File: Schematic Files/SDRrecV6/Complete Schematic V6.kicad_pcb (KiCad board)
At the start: 2 copper layers, 99.6 x 99.7 mm, 74 parts, among them J1 Conn_Coaxial, J2 SJ1-3525N, U1 Si5351A-B-GT, U2 SN74CBT3253, U3 LT6231, U4 LM4562MA, Y1 Crystal_GND24_Small

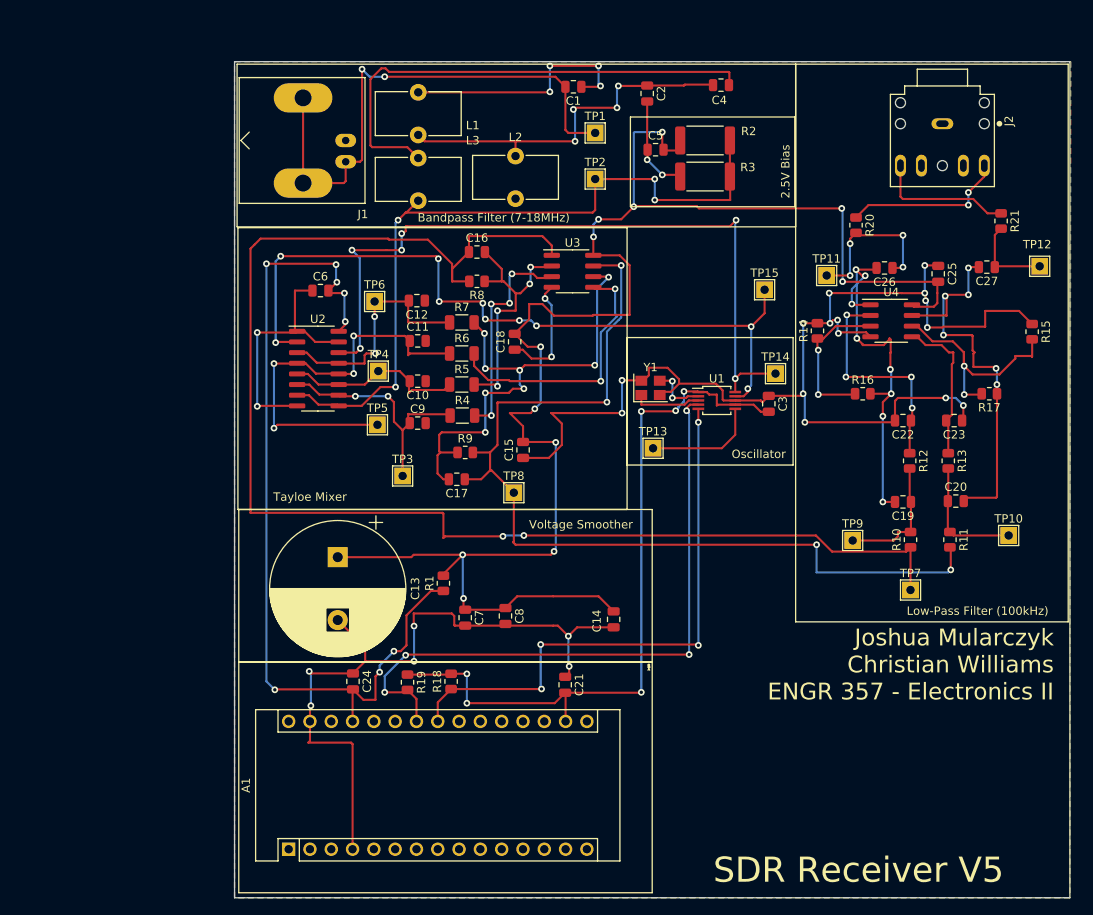
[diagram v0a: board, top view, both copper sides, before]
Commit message: Updated V6 Board
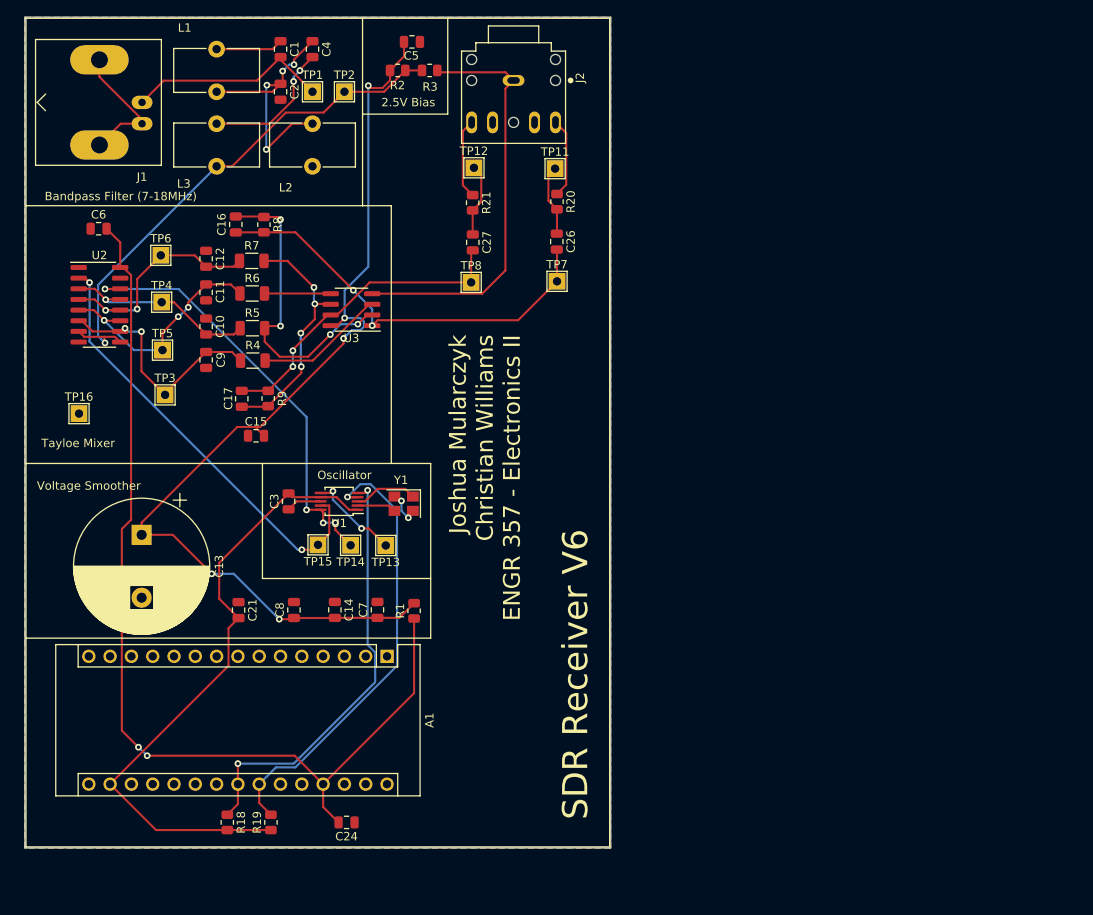
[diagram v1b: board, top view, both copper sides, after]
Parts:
- removed C18, C25: 0.1u, Capacitor_SMD:C_0805_2012Metric
- removed C19, C20, C22, C23: 100p, Capacitor_SMD:C_0805_2012Metric
- removed R10, R11: 4.64k, Resistor_SMD:R_0805_2012Metric
- removed R12, R13: 52.3k, Resistor_SMD:R_0805_2012Metric
- removed R14, R15: 2.49k, Resistor_SMD:R_0805_2012Metric
- removed R16, R17: 17.4k, Resistor_SMD:R_0805_2012Metric
- removed TP10, TP9: TestPoint, TestPoint:TestPoint_THTPad_2.0x2.0mm_Drill1.0mm
- removed U4: LM4562MA, Package_SO:SOIC-8_3.9x4.9mm_P1.27mm
- added TP16: TestPoint, TestPoint:TestPoint_THTPad_2.0x2.0mm_Drill1.0mm, F.Cu at (82.7, 98.1)
- R2, R3: footprint Resistor_SMD:R_2512_6332Metric -> Resistor_SMD:R_0805_2012Metric
- moved TP12 68.5 mm to (129.7, 68.8)
- moved R21 63.0 mm to (129.6, 72.9)
- moved C27 61.4 mm to (129.6, 77.7), turned to -90 degrees
- moved TP15 61.3 mm to (111.2, 113.7), turned to 180 degrees
- moved C3 58.4 mm to (107.6, 108.5), turned to 90 degrees
- moved TP7 56.0 mm to (139.6, 82.3)
- moved TP14 54.6 mm to (115.0, 113.8), turned to 180 degrees
- moved J2 51.4 mm to (134.5, 58.3)
- moved C4 48.9 mm to (110.5, 54.6), turned to -90 degrees
- moved U1 46.6 mm to (113.7, 108.5), turned to 180 degrees
- moved C2 43.7 mm to (106.7, 59.7)
- moved C21 39.9 mm to (101.7, 121.5)
- moved C26 39.2 mm to (139.6, 77.6), turned to -90 degrees
- moved R2 37.6 mm to (120.7, 57.1)
- moved R20 35.8 mm to (139.6, 72.8)
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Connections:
- C26 pad 2: Net-(C19-Pad2) -> Net-(C16-Pad1)
- C27 pad 2: Net-(C20-Pad2) -> Net-(C17-Pad1)
- J1 pad 1: GND -> Net-(C1-Pad2)
- J1 pad 2: Net-(C1-Pad2) -> GND
- J2 pad 10: (no net) -> unconnected-(J2-Pad10)
- J2 pad 11: (no net) -> unconnected-(J2-Pad11)
- U2 pad 11: Net-(C10-Pad2) -> Net-(C11-Pad1)
- U2 pad 12: Net-(C11-Pad1) -> Net-(C12-Pad2)
- U2 pad 13: Net-(C12-Pad2) -> Net-(C10-Pad2)
- U2 pad 3: Net-(C12-Pad2) -> Net-(C10-Pad2)
- U2 pad 4: Net-(C11-Pad1) -> Net-(C12-Pad2)
- U2 pad 5: Net-(C10-Pad2) -> Net-(C11-Pad1)
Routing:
- net GND: track 274.8 -> 74.2 mm, vias 27 -> 2
- net Net-(C16-Pad1): track 167.1 -> 50.1 mm
- net Net-(C17-Pad1): track 115.8 -> 37.8 mm, vias 4 -> 2
- net Filtered 5V: track 196.6 -> 119.3 mm, vias 12 -> 5
- net Net-(C20-Pad2): track 49.4 -> 0.00 mm, vias 6 -> 0
- net Net-(C19-Pad2): track 47.1 -> 0.00 mm, vias 8 -> 0
- net Net-(C4-Pad2): track 59.3 -> 16.4 mm, vias 0 -> 2
- net Net-(C1-Pad2): track 64.5 -> 24.5 mm, vias 2 -> 0
- net Net-(TP15-Pad1): track 91.3 -> 52.6 mm, vias 10 -> 2
- net Net-(TP14-Pad1): track 89.3 -> 51.5 mm, vias 6 -> 4
- net Net-(C17-Pad2): track 58.5 -> 28.9 mm, vias 8 -> 4
- net Net-(R15-Pad2): track 28.2 -> 0.00 mm, vias 2 -> 0
- net Net-(C22-Pad1): track 27.3 -> 0.00 mm, vias 4 -> 0
- net Net-(L3-Pad2): track 88.7 -> 62.7 mm, vias 4 -> 1
- net Net-(R6-Pad2): track 31.9 -> 7.91 mm, vias 2 -> 0
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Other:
- board size 99.6 x 99.7 mm -> 69.9 x 99.1 mm
- board text added: "SDR Receiver V6"
- board text removed: "Low-Pass Filter (100kHz)"
- board text removed: "SDR Receiver V5"
